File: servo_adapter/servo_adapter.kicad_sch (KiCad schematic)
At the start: 11 parts, among them J1 T4140012081-000, J2 Conn_01x10_Socket, Q1 MUN5233, Q2 MUN5233, Q3 MUN5233, Q4 MUN5233

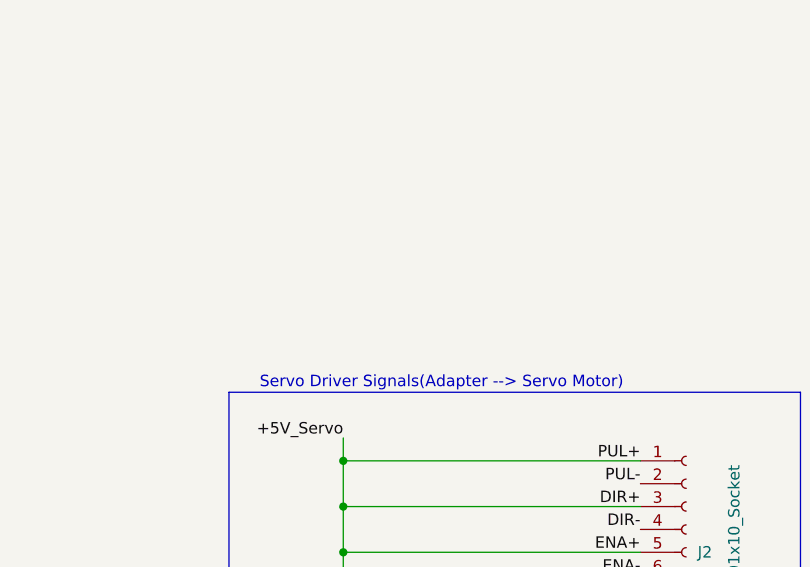
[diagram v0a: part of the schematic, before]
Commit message: Updated with generic 2pin symbol and labels used for the servo motor power connection.
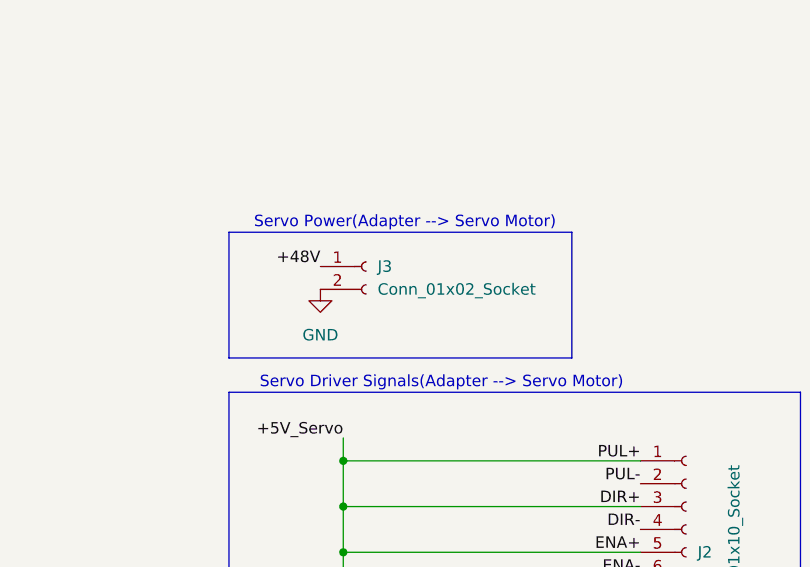
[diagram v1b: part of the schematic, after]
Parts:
- added J3: Conn_01x02_Socket, symbol Connector:Conn_01x02_Socket
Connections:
- net GND: now also J3.2 (Pin_2)
- new net +48V: J3.1 (Pin_1)
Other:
- note added: "Servo Power(Adapter --> Servo Motor)"
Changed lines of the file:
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@@
+	)
+	(rectangle
+		(start 165.1 40.64)
+		(end 203.2 54.61)
+		(stroke
+			(width 0)
+			(type default)
+		)
+		(fill
+			(type none)
+		)
 	)
 	(rectangle
@@
 		(exclude_from_sim no)
 		(at 25.654 67.564 0)
+		(effects
+			(font
+				(size 1.27 1.27)
+			)
+		)
+	)
+	(text "Servo Power(Adapter --> Servo Motor)"
+		(exclude_from_sim no)
+		(at 184.658 39.624 0)
 		(effects
 			(font
@@
 			)
 			(justify left bottom)
+		)
+	)
+	(label "+48V"
+		(at 175.26 44.45 180)
+		(effects
+			(font
+				(size 1.27 1.27)
+			)
+			(justify right bottom)
 		)
 	)
@@
 	)
 	(symbol
+		(lib_id "Connector:Conn_01x02_Socket")
+		(at 180.34 44.45 0)
+		(unit 1)
+		(exclude_from_sim no)
+		(in_bom yes)
+		(on_board yes)
+		(dnp no)
+		(fields_autoplaced yes)
+		(property "Reference" "J3"
+			(at 181.61 44.4499 0)
+			(effects
+				(font
+					(size 1.27 1.27)
+				)
+				(justify left)
+			)
+		)
+		(property "Value" "Conn_01x02_Socket"
+			(at 181.61 46.9899 0)
+			(effects
+				(font
+					(size 1.27 1.27)
+				)
+				(justify left)
+			)
+		)
+		(property "Footprint" ""
+			(at 180.34 44.45 0)
+			(effects
+				(font
+					(size 1.27 1.27)
+				)
+				(hide yes)
+			)
+		)
+		(property "Datasheet" "~"
+			(at 180.34 44.45 0)
+			(effects
+				(font
+					(size 1.27 1.27)
+				)
+				(hide yes)
+			)
+		)
+		(property "Description" "Generic connector, single row, 01x02, script generated"
+			(at 180.34 44.45 0)
+			(effects
+				(font
+					(size 1.27 1.27)
+				)
+				(hide yes)
+			)
+		)
+		(pin "2"
+		)
+		(pin "1"
+		)
+		(instances
+			(project ""
+				(path "/d2a6932a-1682-4170-bbbb-2fb2c0f935d7"
+					(reference "J3")
+					(unit 1)
+				)
+			)
+		)
+	)
+	(symbol
 		(lib_id "T4140012081-000:T4140012081-000")
 		(at 40.64 30.48 0)
@@
 					(unit 1)
 				)
+			)
+		)
+	)
+	(symbol
+		(lib_id "power:GND")
+		(at 175.26 46.99 0)
+		(unit 1)
+		(exclude_from_sim no)
+		(in_bom yes)
+		(on_board yes)
+		(dnp no)
+		(fields_autoplaced yes)
+		(property "Reference" "#PWR04"
+			(at 175.26 53.34 0)
+			(effects
+				(font
+					(size 1.27 1.27)
+				)
+				(hide yes)
+			)
+		)
+		(property "Value" "GND"
+			(at 175.26 52.07 0)
+			(effects
+				(font
+					(size 1.27 1.27)
+				)
+			)
+		)
+		(property "Footprint" ""
+			(at 175.26 46.99 0)
+			(effects
+				(font
+					(size 1.27 1.27)
+				)
+				(hide yes)
+			)
+		)
+		(property "Datasheet" ""
+			(at 175.26 46.99 0)
+			(effects
+				(font
+					(size 1.27 1.27)
+				)
+				(hide yes)
+			)
+		)
+		(property "Description" "Power symbol creates a global label with name \"GND\" , ground"
+			(at 175.26 46.99 0)
+			(effects
+				(font
+					(size 1.27 1.27)
+				)
+				(hide yes)
+			)
+		)
+		(pin "1"
+		)
+		(instances
+			(project "servo_adapter"
+				(path "/d2a6932a-1682-4170-bbbb-2fb2c0f935d7"
+					(reference "#PWR04")
+					(unit 1)
+				)

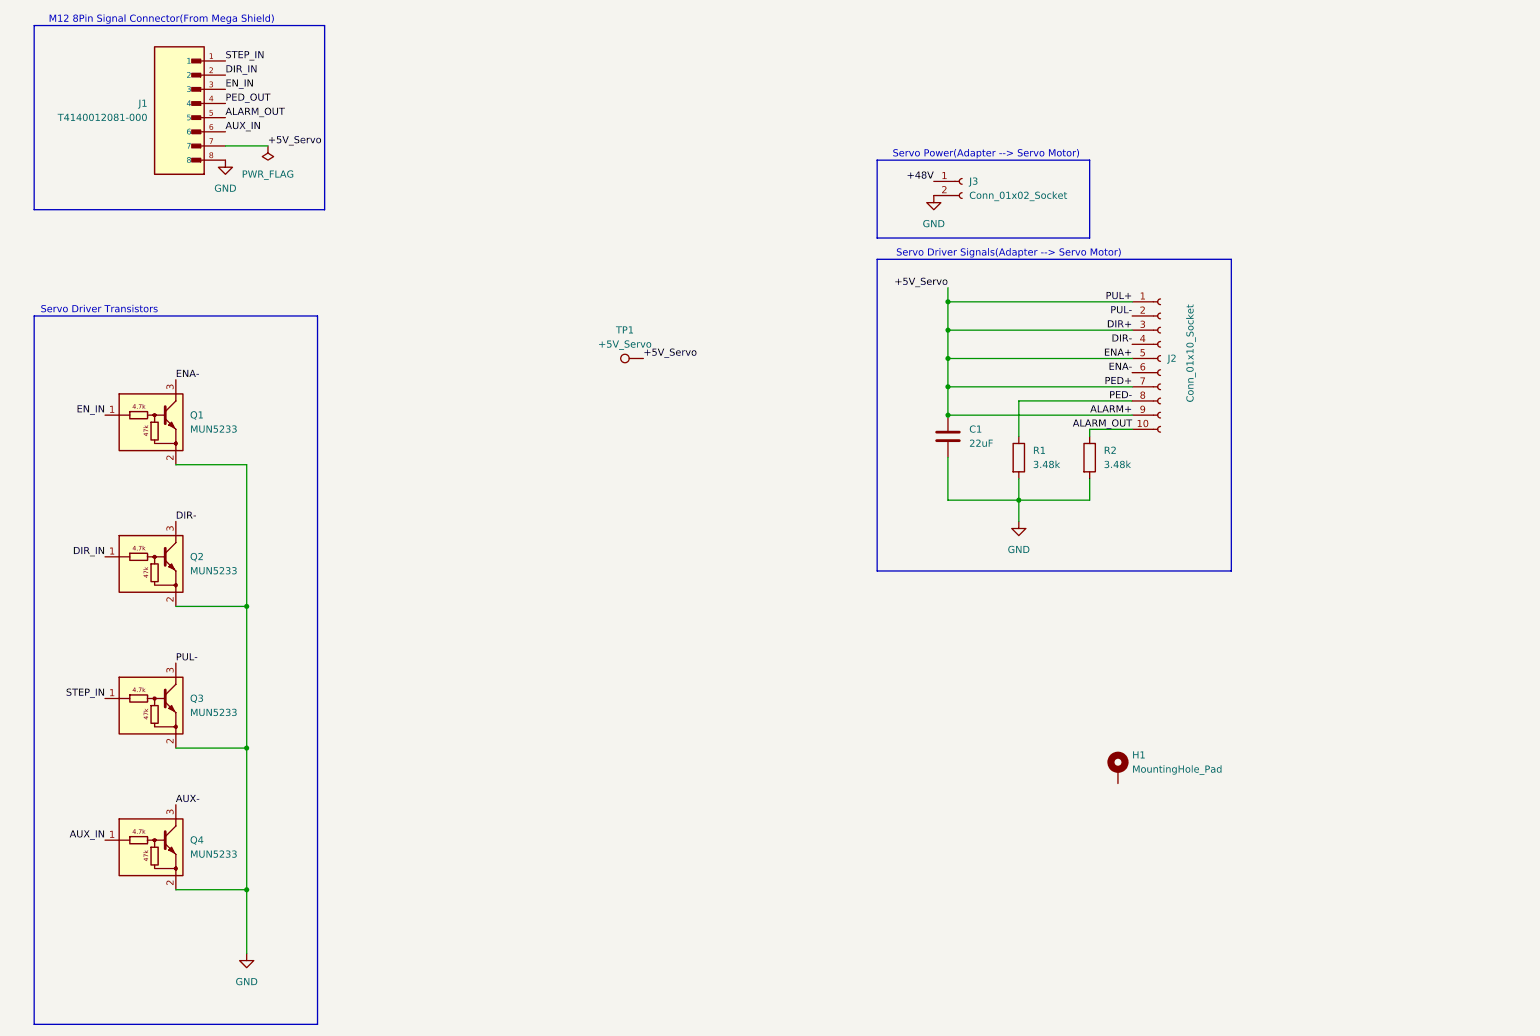
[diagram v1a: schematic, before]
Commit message: Added mounting holes and Test Points.
Added a second mounting hole. Added test points for +48VDC, +5VDC and
GND.
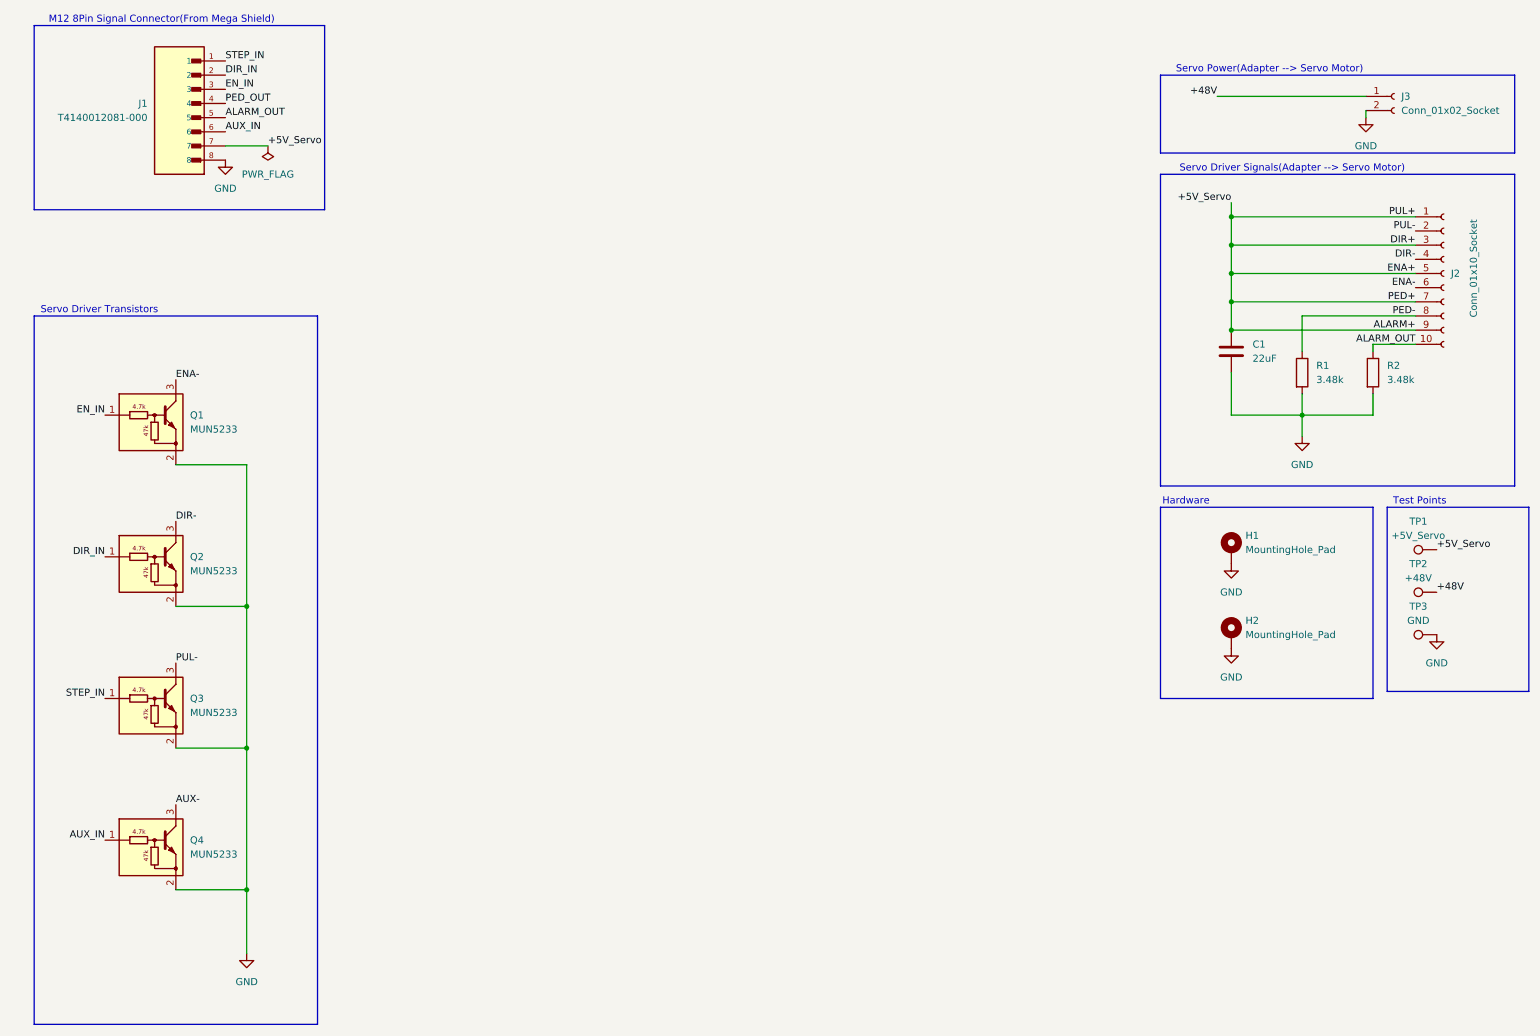
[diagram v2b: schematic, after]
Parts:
- added H2: MountingHole_Pad, symbol Mechanical:MountingHole_Pad
- added TP2: +48V, symbol Connector:TestPoint
- added TP3: GND, symbol Connector:TestPoint
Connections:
- net +48V: now also TP2.1
- net GND: now also H1.1, H2.1, TP3.1
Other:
- note added: "Hardware"
- note added: "Test Points"
- moved on the sheet: C1, H1, J2, J3, R1, R2, TP1
